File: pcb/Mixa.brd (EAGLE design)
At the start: 109.2 x 39.6 mm, 51 parts

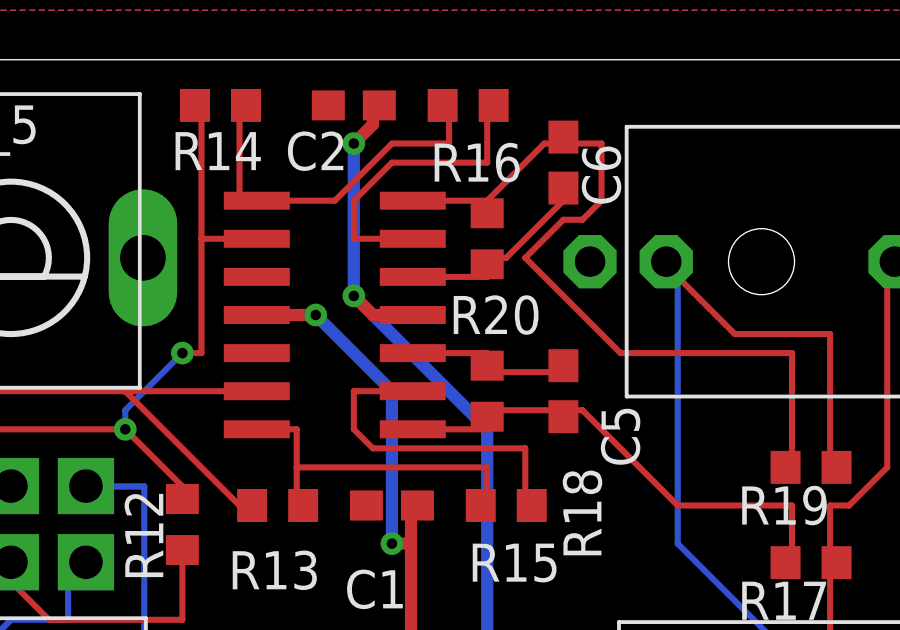
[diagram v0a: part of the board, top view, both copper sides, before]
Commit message: bug fix, feedback in second stage must go to -, GND to + inputs
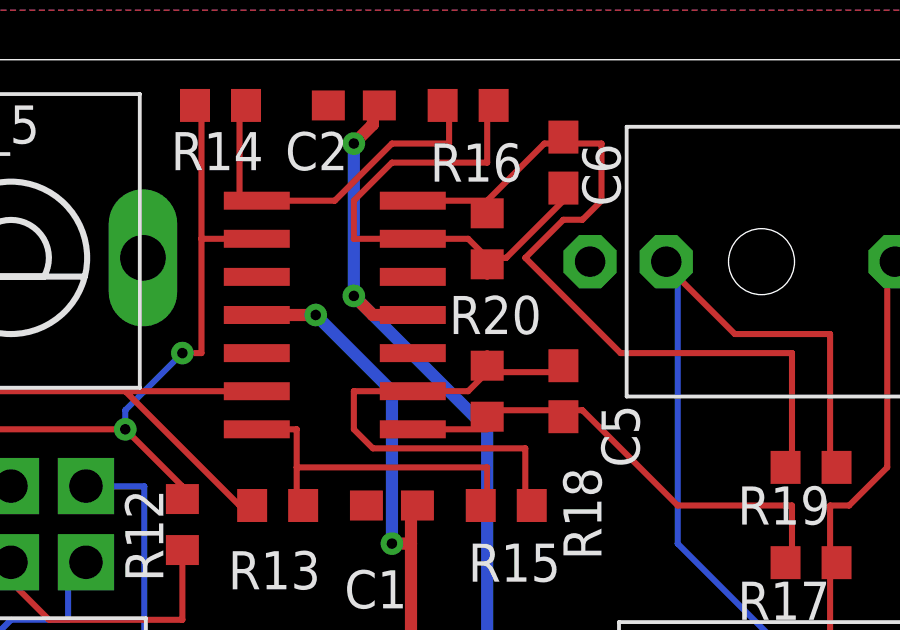
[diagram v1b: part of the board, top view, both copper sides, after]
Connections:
- removed net N$15: OPAMP_IS.13, R16.2
- removed net N$16: OPAMP_IS.9, R15.2
- net GND: now also OPAMP_IS.10, OPAMP_IS.12
- net N$13: now also OPAMP_IS.13, R16.2; no longer OPAMP_IS.12
- net N$7: now also OPAMP_IS.9, R15.2; no longer OPAMP_IS.10
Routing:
- net N$7: track 5.87 -> 17.5 mm
- net N$16: track 11.3 -> 0.00 mm
- net N$13: track 6.86 -> 17.5 mm
- net N$15: track 10.3 -> 0.00 mm
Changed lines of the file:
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@@
 <contactref element="OPAMP_IS" pad="3"/>
 <contactref element="OPAMP_IS" pad="5"/>
+<contactref element="OPAMP_IS" pad="10"/>
+<contactref element="OPAMP_IS" pad="12"/>
 </signal>
 <signal name="VSS" class="1">
@@
 </signal>
 <signal name="N$7">
-<contactref element="OPAMP_IS" pad="10"/>
 <contactref element="R18" pad="1"/>
 <contactref element="C5" pad="2"/>
 <wire x1="94.615" y1="14.605" x2="92.075" y2="14.605" width="0.2032" layer="1"/>
+<wire x1="94.615" y1="14.605" x2="94.615" y2="14.82" width="0.2032" layer="1"/>
+<wire x1="92.075" y1="15.24" x2="92.075" y2="14.82" width="0.2032" layer="1"/>
+<contactref element="R15" pad="2"/>
+<contactref element="OPAMP_IS" pad="9"/>
+<wire x1="93.345" y1="12.065" x2="93.345" y2="10.16" width="0.2032" layer="1"/>
+<wire x1="88.265" y1="12.065" x2="93.345" y2="12.065" width="0.2032" layer="1"/>
+<wire x1="87.63" y1="12.7" x2="88.265" y2="12.065" width="0.2032" layer="1"/>
+<wire x1="87.63" y1="13.97" x2="87.63" y2="12.7" width="0.2032" layer="1"/>
+<wire x1="89.595" y1="13.97" x2="87.63" y2="13.97" width="0.2032" layer="1"/>
+<wire x1="93.345" y1="10.16" x2="93.56" y2="10.16" width="0.2032" layer="1"/>
+<wire x1="91.44" y1="13.97" x2="92.075" y2="14.605" width="0.2032" layer="1"/>
+<wire x1="89.595" y1="13.97" x2="91.44" y2="13.97" width="0.2032" layer="1"/>
 <wire x1="92.075" y1="14.605" x2="92.075" y2="14.82" width="0.2032" layer="1"/>
-<wire x1="94.615" y1="14.605" x2="94.615" y2="14.82" width="0.2032" layer="1"/>
-<wire x1="89.595" y1="15.24" x2="92.075" y2="15.24" width="0.2032" layer="1"/>
-<wire x1="92.075" y1="15.24" x2="92.075" y2="14.82" width="0.2032" layer="1"/>
 </signal>
 <signal name="N$13">
-<contactref element="OPAMP_IS" pad="12"/>
 <contactref element="R20" pad="1"/>
 <contactref element="C6" pad="2"/>
-<wire x1="89.595" y1="17.78" x2="92.075" y2="17.78" width="0.2032" layer="1"/>
 <wire x1="92.075" y1="17.78" x2="92.075" y2="18.2" width="0.2032" layer="1"/>
 <wire x1="92.71" y1="18.415" x2="94.615" y2="20.32" width="0.2032" layer="1"/>
 <wire x1="92.075" y1="18.415" x2="92.71" y2="18.415" width="0.2032" layer="1"/>
 <wire x1="94.615" y1="20.32" x2="94.615" y2="20.74" width="0.2032" layer="1"/>
-<wire x1="92.075" y1="18.415" x2="92.075" y2="18.2" width="0.2032" layer="1"/>
-</signal>
-<signal name="N$15">
 <contactref element="R16" pad="2"/>
 <contactref element="OPAMP_IS" pad="13"/>
@@
 <wire x1="89.595" y1="19.05" x2="87.63" y2="19.05" width="0.2032" layer="1"/>
 <wire x1="92.075" y1="23.495" x2="92.29" y2="23.495" width="0.2032" layer="1"/>
-</signal>
-<signal name="N$16">
-<contactref element="R15" pad="2"/>
-<contactref element="OPAMP_IS" pad="9"/>
-<wire x1="93.345" y1="12.065" x2="93.345" y2="10.16" width="0.2032" layer="1"/>
-<wire x1="88.265" y1="12.065" x2="93.345" y2="12.065" width="0.2032" layer="1"/>
-<wire x1="87.63" y1="12.7" x2="88.265" y2="12.065" width="0.2032" layer="1"/>
-<wire x1="87.63" y1="13.97" x2="87.63" y2="12.7" width="0.2032" layer="1"/>
-<wire x1="89.595" y1="13.97" x2="87.63" y2="13.97" width="0.2032" layer="1"/>
-<wire x1="93.345" y1="10.16" x2="93.56" y2="10.16" width="0.2032" layer="1"/>
+<wire x1="91.44" y1="19.05" x2="92.075" y2="18.415" width="0.2032" layer="1"/>
+<wire x1="89.595" y1="19.05" x2="91.44" y2="19.05" width="0.2032" layer="1"/>
+<wire x1="92.075" y1="18.415" x2="92.075" y2="18.2" width="0.2032" layer="1"/>
 </signal>
 </signals>
